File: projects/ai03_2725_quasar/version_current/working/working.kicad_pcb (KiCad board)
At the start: 2 copper layers, 170 x 50 mm, 34 parts, among them J1 Conn_01x16, J2 Conn_01x08, J3 Conn_01x01, J4 USB_B, J5 Solenoid, Q1 Q_NMOS_GSD, SW1 SW_Push, U1 ATmega32U4-AU, U2 PRTR5V0U2X, Y1 16Mhz

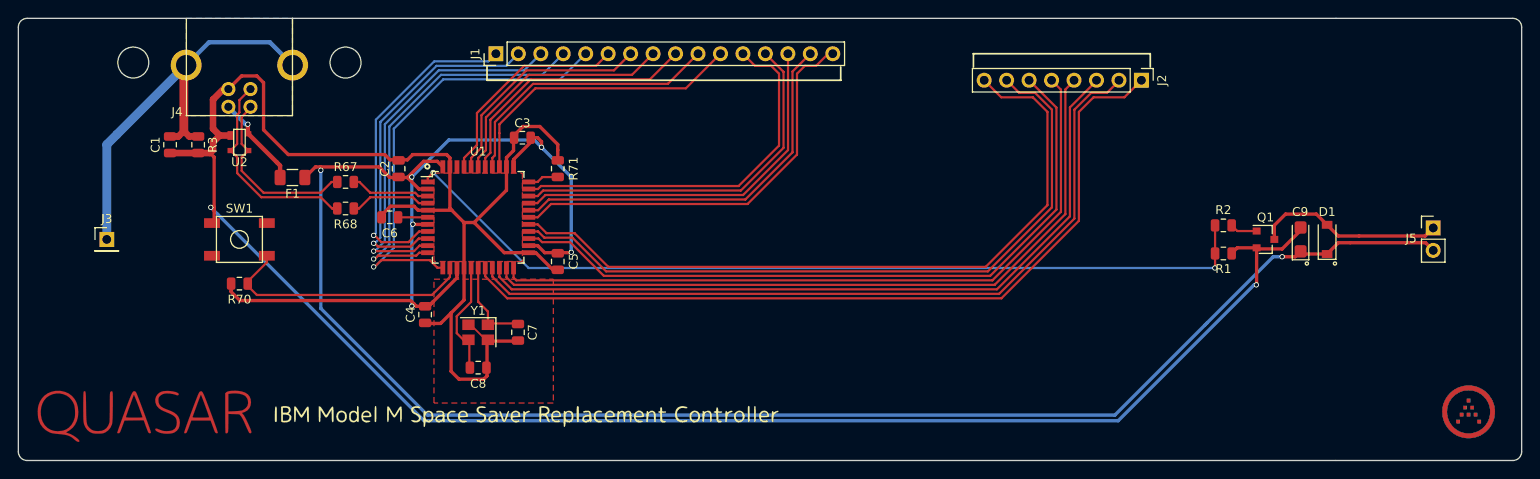
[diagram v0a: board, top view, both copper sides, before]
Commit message: updated all projects from src
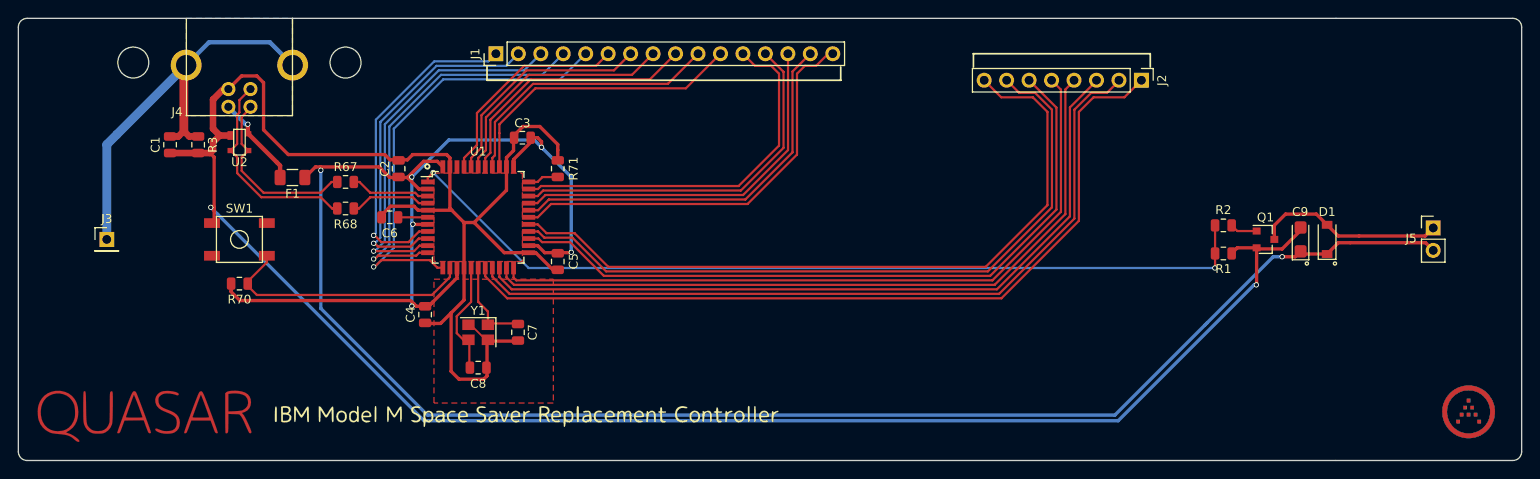
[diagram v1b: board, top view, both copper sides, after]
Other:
- net class Default added: clearance 0.2032, trace_width 0.254, via_dia 0.6, via_drill 0.4
- net class Earth added: clearance 0.2032, trace_width 0.5, via_dia 0.6, via_drill 0.4
- net class Power added: clearance 0.2032, trace_width 0.381, via_dia 0.6, via_drill 0.4
